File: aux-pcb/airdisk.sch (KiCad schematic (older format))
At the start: 52 parts, among them U1 USBLC6-2SC6

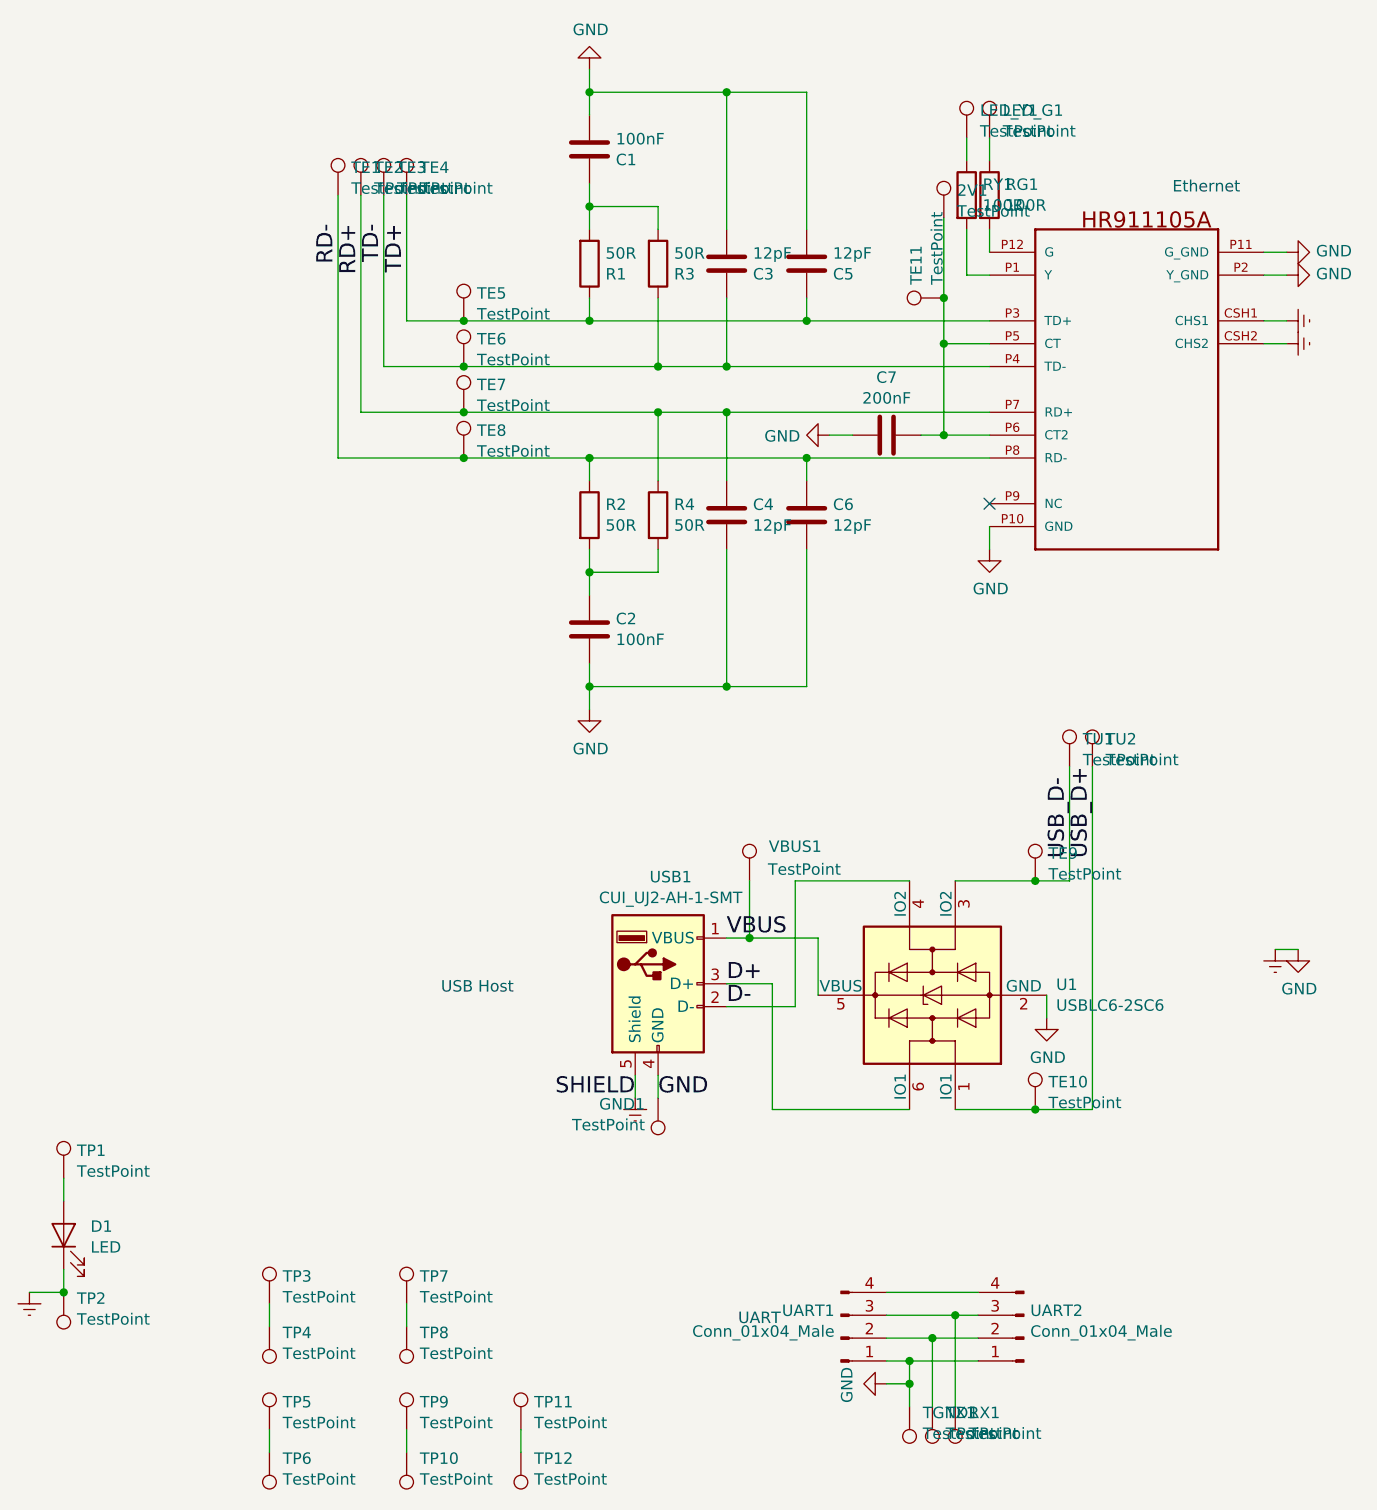
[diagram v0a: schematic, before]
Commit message: update pcb
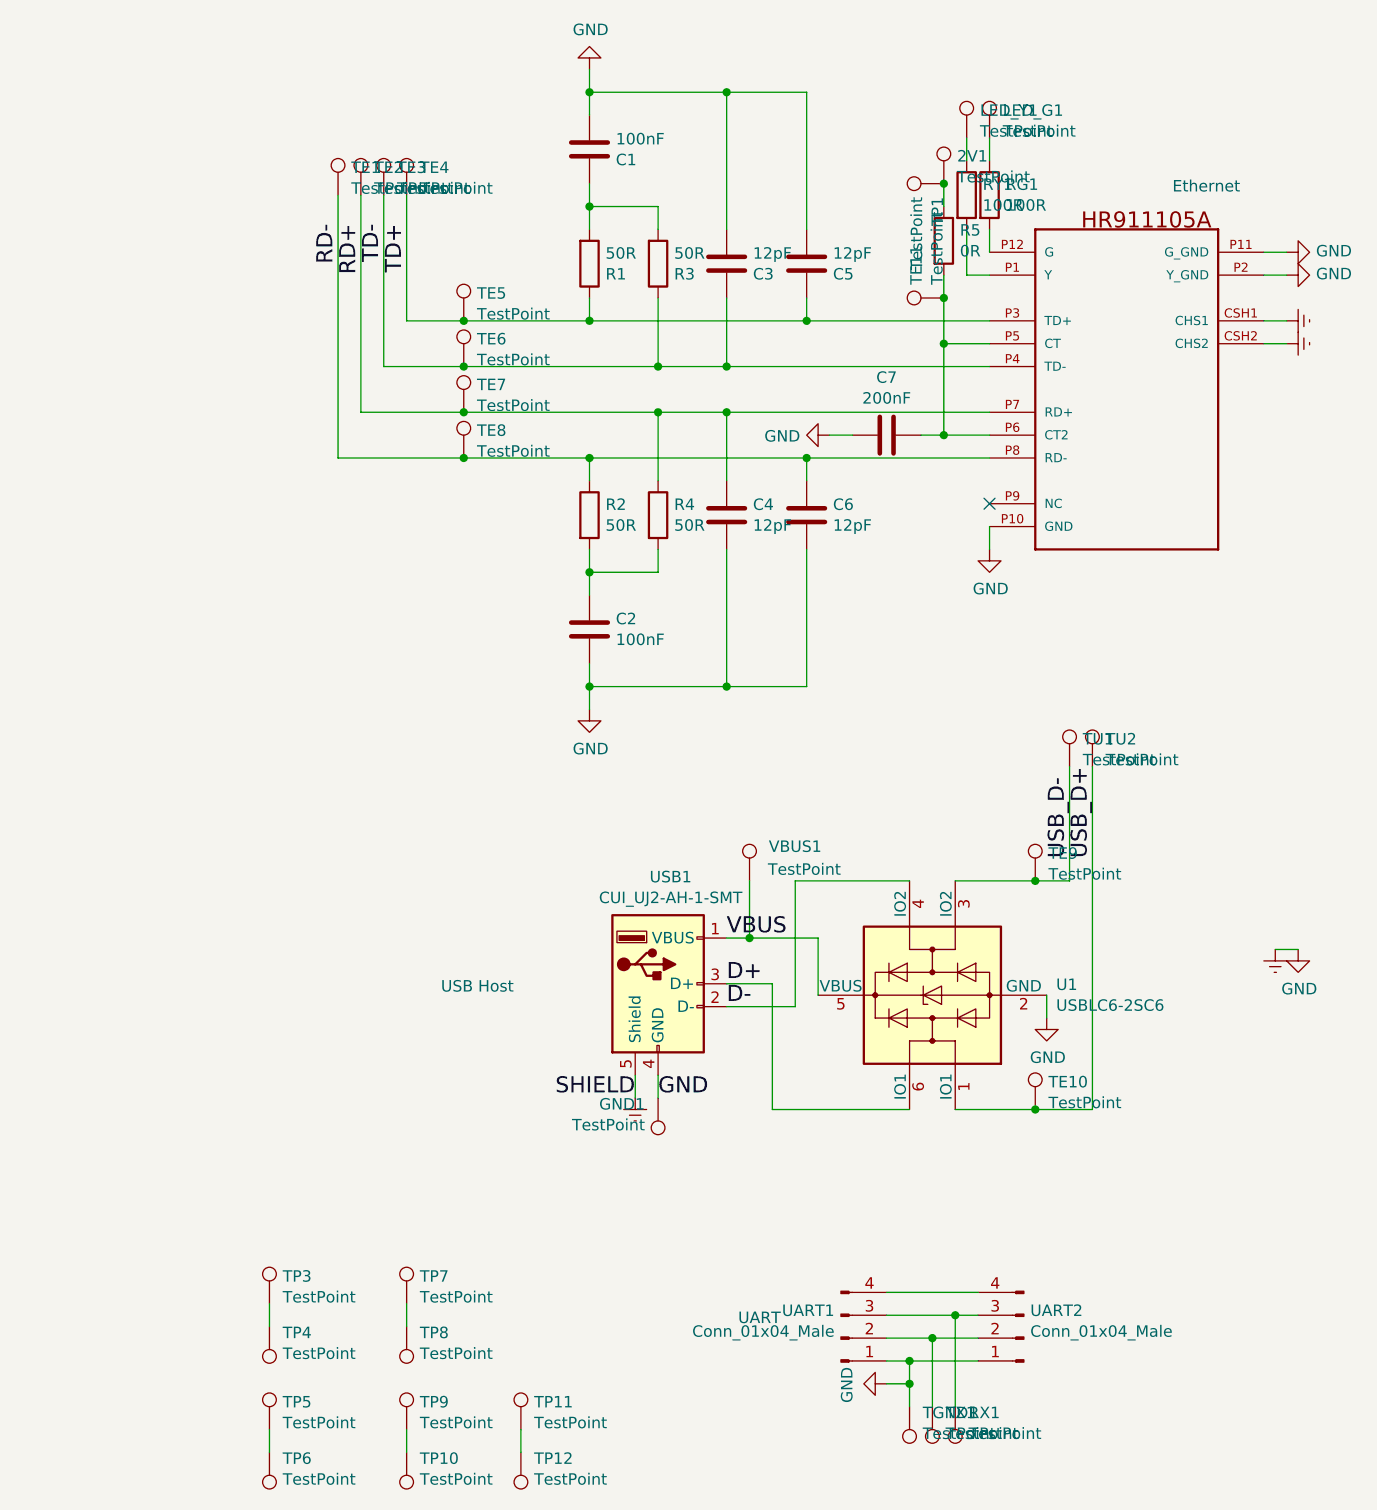
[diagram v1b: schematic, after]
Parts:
- removed D1: LED, Diode_SMD:D_0603_1608Metric_Pad1.05x0.95mm_HandSolder, symbol Device:LED
- removed TP2: TestPoint, airdisk:TE_3-2199250-5, symbol Connector:TestPoint
- added R5: 0R, Resistor_SMD:R_0402_1005Metric, symbol Device:R
- TP1: footprint airdisk:TE_3-2199250-5 -> TestPoint:TestPoint_Pad_D1.5mm
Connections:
- net at C7.1, ETH1.P5 (CT), ETH1.P6 (CT2)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: now also R5.2; no longer 2V1.1
- net at TP1.1: now also 2V1.1, R5.1
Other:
- moved on the sheet: 2V1
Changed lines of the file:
@@
 EESchema Schematic File Version 4
 LIBS:airdisk-cache
-EELAYER 26 0
+EELAYER 29 0
 EELAYER END
 $Descr A4 11693 8268
@@
 Wire Wire Line
 	6050 3100 6050 3200
-Wire Wire Line
-	5850 1750 5850 2100
 $Comp
 L power:GND #PWR0109
@@
 L Connector:TestPoint 2V1
 U 1 1 5D0EF73D
-P 5850 1750
-F 0 "2V1" H 5908 1870 50  0000 L CNN
-F 1 "TestPoint" H 5908 1779 50  0000 L CNN
-F 2 "airdisk:TE_3-2199250-5" H 6050 1750 50  0001 C CNN
-F 3 "~" H 6050 1750 50  0001 C CNN
-	1    5850 1750
-	1    0    0    -1
-$EndComp
-$Comp
-L Connector:TestPoint TP1
-U 1 1 5D125817
-P 2000 5950
-F 0 "TP1" H 2058 6070 50  0000 L CNN
-F 1 "TestPoint" H 2058 5979 50  0000 L CNN
-F 2 "airdisk:TE_3-2199250-5" H 2200 5950 50  0001 C CNN
-F 3 "~" H 2200 5950 50  0001 C CNN
-	1    2000 5950
-	1    0    0    -1
-$EndComp
-Wire Wire Line
-	2000 5950 2000 6050
-$Comp
-L Device:LED D1
-U 1 1 5D127CD8
-P 2000 6200
-F 0 "D1" V 2038 6083 50  0000 R CNN
-F 1 "LED" V 1947 6083 50  0000 R CNN
-F 2 "Diode_SMD:D_0603_1608Metric_Pad1.05x0.95mm_HandSolder" H 2000 6200 50  0001 C CNN
-F 3 "~" H 2000 6200 50  0001 C CNN
-	1    2000 6200
-	0    -1   -1   0
-$EndComp
-$Comp
-L Connector:TestPoint TP2
-U 1 1 5D1280AE
-P 2000 6450
-F 0 "TP2" H 1942 6477 50  0000 R CNN
-F 1 "TestPoint" H 1942 6568 50  0000 R CNN
-F 2 "airdisk:TE_3-2199250-5" H 2200 6450 50  0001 C CNN
-F 3 "~" H 2200 6450 50  0001 C CNN
-	1    2000 6450
-	-1   0    0    1
-$EndComp
-Wire Wire Line
-	2000 6350 2000 6450
+P 5850 1600
+F 0 "2V1" H 5908 1720 50  0000 L CNN
+F 1 "TestPoint" H 5908 1629 50  0000 L CNN
+F 2 "airdisk:TE_3-2199250-5" H 6050 1600 50  0001 C CNN
+F 3 "~" H 6050 1600 50  0001 C CNN
+	1    5850 1600
+	1    0    0    -1
+$EndComp
 $Comp
 L Connector:TestPoint TP3
@@
 	0    -1   1    0
 $EndComp
+Wire Wire Line
+	5850 2100 5850 2300
+$Comp
+L Device:R R5
+U 1 1 5D276C22
+P 5850 1850
+F 0 "R5" H 5920 1896 50  0000 L CNN
+F 1 "0R" H 5920 1805 50  0000 L CNN
+F 2 "Resistor_SMD:R_0402_1005Metric" V 5780 1850 50  0001 C CNN
+F 3 "~" H 5850 1850 50  0001 C CNN
+	1    5850 1850
+	1    0    0    -1
+$EndComp
+Wire Wire Line
+	5850 1600 5850 1700
+Wire Wire Line
+	5850 2000 5850 2100
 Connection ~ 5850 2100
-Wire Wire Line
-	5850 2100 5850 2300
-$Comp
-L power:Earth #PWR0102
-U 1 1 5D176C8B
-P 1850 6450
-F 0 "#PWR0102" H 1850 6200 50  0001 C CNN
-F 1 "Earth" H 1850 6300 50  0001 C CNN
-F 2 "" H 1850 6450 50  0001 C CNN
-F 3 "~" H 1850 6450 50  0001 C CNN
-	1    1850 6450
-	1    0    0    -1
-$EndComp
-Wire Wire Line
-	1850 6450 2000 6450
-Connection ~ 2000 6450
+$Comp
+L Connector:TestPoint TP1
+U 1 1 5D290D82
+P 5850 1600
+F 0 "TP1" H 5792 1627 50  0000 R CNN
+F 1 "TestPoint" H 5792 1718 50  0000 R CNN
+F 2 "TestPoint:TestPoint_Pad_D1.5mm" H 6050 1600 50  0001 C CNN
+F 3 "~" H 6050 1600 50  0001 C CNN
+	1    5850 1600
+	0    -1   -1   0
+$EndComp
+Connection ~ 5850 1600
 $EndSCHEMATC
